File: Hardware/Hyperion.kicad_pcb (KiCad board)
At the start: 2 copper layers, 90.2 x 95.9 mm, 41 parts, among them J1 USB, J2 CONN-DC, Q1 MOSFET-P, Q2 FDC6561, U1 FT2232H, U2 93LC46/OT, U3 LTC4361-T, X1 12MHz

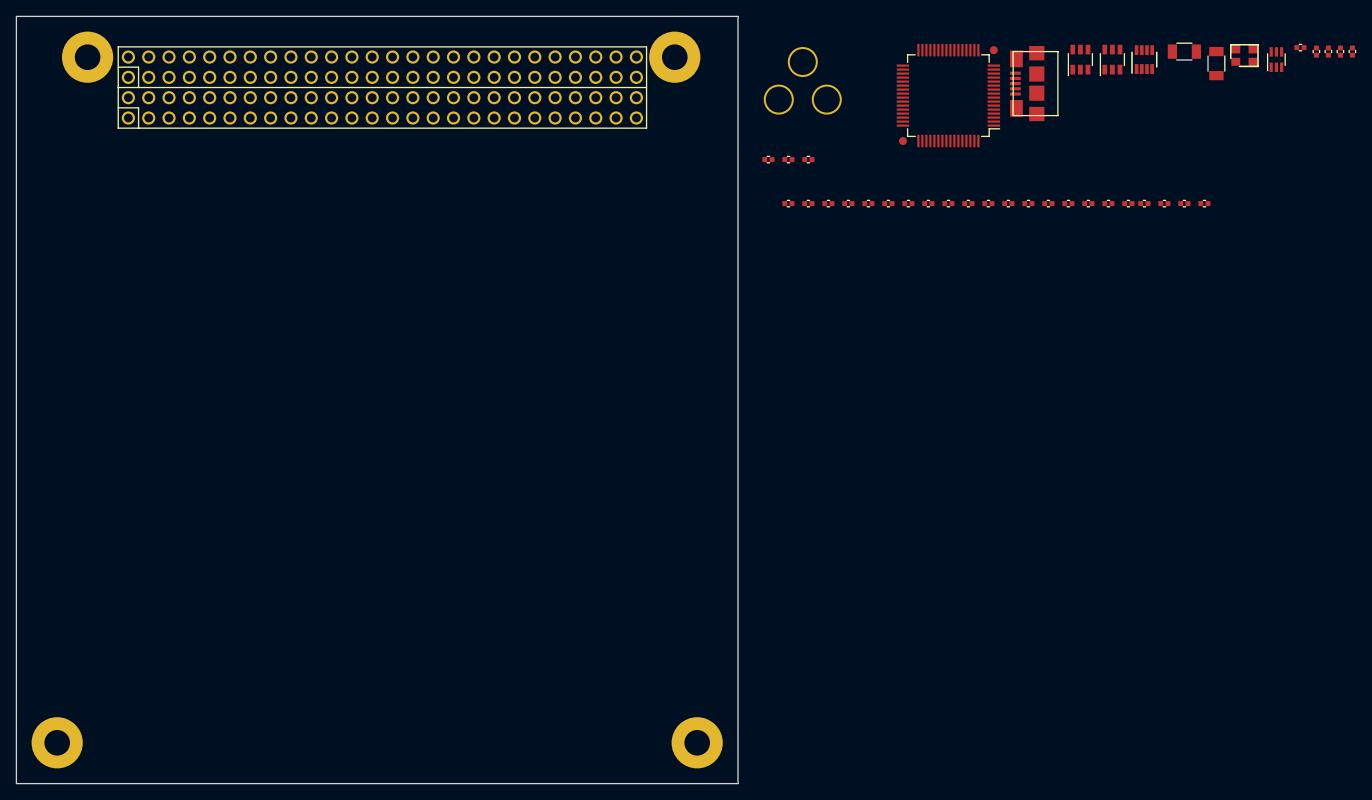
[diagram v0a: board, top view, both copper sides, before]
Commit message: Core support circuitry
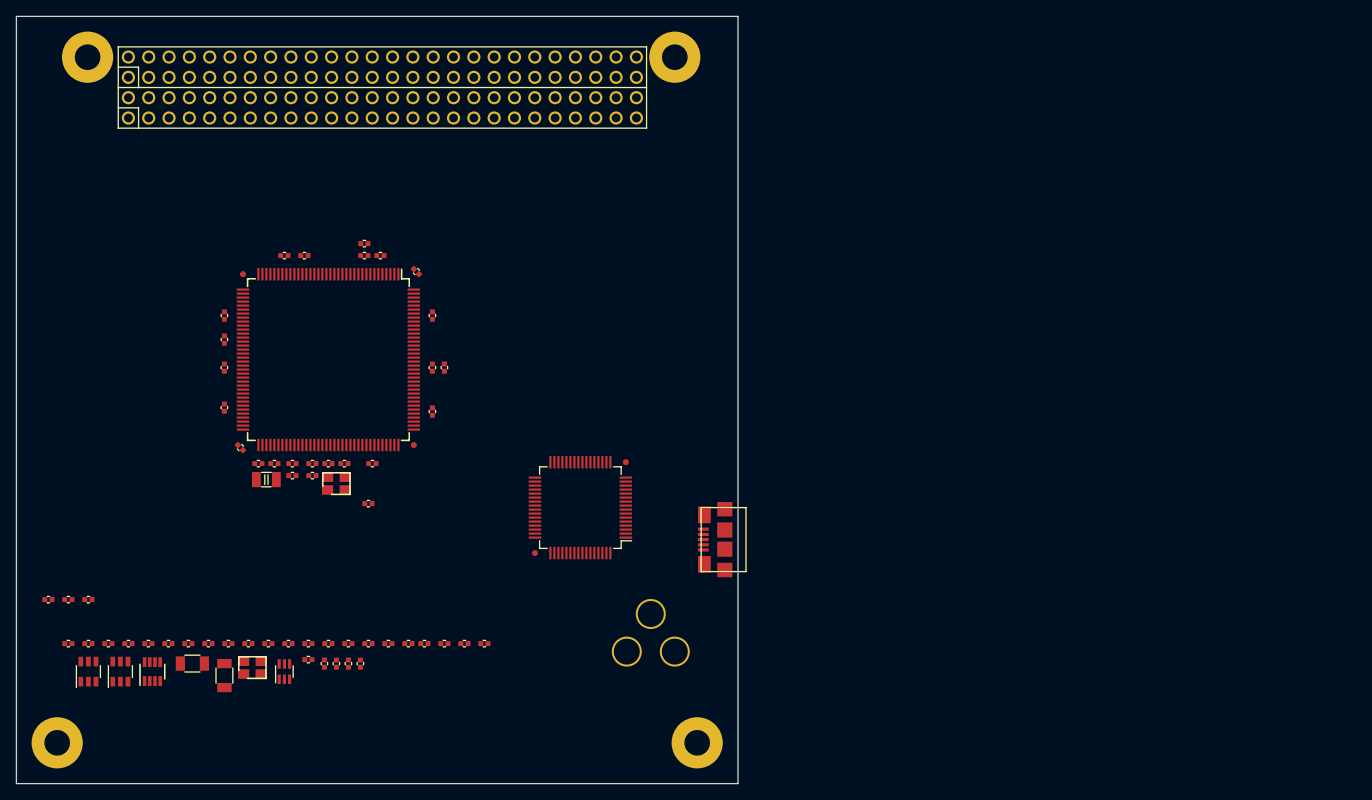
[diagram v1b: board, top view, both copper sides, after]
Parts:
- added C17: 0.1uF, CAPC1005-N, F.Cu at (145.5, 79.0)
- added C18: 0.1uF, CAPC1005-N, F.Cu at (136.0, 79.0)
- added C19: 0.1uF, CAPC1005-N, F.Cu at (133.5, 79.0)
- added C20: 0.1uF, CAPC1005-N, F.Cu at (126.0, 86.5)
- added C21: 0.1uF, CAPC1005-N, F.Cu at (126.0, 93.0)
- added C22: 0.1uF, CAPC1005-N, F.Cu at (126.0, 98.0)
- added C23: 0.1uF, CAPC1005-N, F.Cu at (134.5, 106.5)
- added C24: 0.1uF, CAPC1005-N, F.Cu at (144.0, 110.0)
- added C25: 0.1uF, CAPC1005-N, F.Cu at (144.5, 105.0)
- added C26: 0.1uF, CAPC1005-N, F.Cu at (152.0, 98.5)
- added C27: 0.1uF, CAPC1005-N, F.Cu at (152.0, 93.0)
- added C28: 0.1uF, CAPC1005-N, F.Cu at (152.0, 86.5)
- added C29: 3.3uF, CAPC1005-N, F.Cu at (150.0, 81.0)
- added C30: 3.3uF, CAPC1005-N, F.Cu at (128.0, 103.0)
- added C31: 0.1uF, CAPC1005-N, F.Cu at (126.0, 89.5)
- added C32: 3.3uF, CAPC1005-N, F.Cu at (153.5, 93.0)
- added C33: 10pF, CAPC1005-N, F.Cu at (139.0, 105.0)
- added C34: 10pF, CAPC1005-N, F.Cu at (130.2, 105.0)
- added C35: 10pF, CAPC1005-N, F.Cu at (141.0, 105.0)
- added C36: 10pF, CAPC1005-N, F.Cu at (132.2, 105.0)
- added C37: 0.1uF, CAPC1005-N, F.Cu at (143.5, 79.0)
- added C38: 0.1uF, CAPC1005-N, F.Cu at (134.5, 105.0)
- added C39: 0.1uF, CAPC1005-N, F.Cu at (137.0, 105.0)
- added FB3: FERRITE, INDC1005-N, F.Cu at (143.5, 77.5)
- added R12: 1k, RESC1005-N, F.Cu at (137.0, 106.5)
- added U4: TM4C123GH6PGE, QFP50P2200X2200-144N, F.Cu at (139.0, 92.0)
- added X2: 12MHz, XTAL-4SMD-32X25, F.Cu at (140.0, 107.5)
- added X3: 32.768kHz, XTAL-2SMD-32x15, F.Cu at (131.2, 107.0)
- C11, C14: value 27pF -> 10pF
- moved C16 145.7 mm to (136.5, 129.5)
- moved D1 145.7 mm to (141.5, 130.0)
- moved D2 145.7 mm to (143.0, 130.0)
- moved Q1 145.7 mm to (133.5, 131.0)
- moved Q2 145.7 mm to (109.0, 131.0)
- moved R1 145.7 mm to (138.5, 130.0)
- moved R11 145.7 mm to (122.0, 130.0)
- moved R2 145.7 mm to (140.0, 130.0)
- moved TH1 145.7 mm to (126.0, 131.5)
- moved U2 145.7 mm to (113.0, 131.0)
- moved U3 145.7 mm to (117.0, 131.0)
- moved X1 145.7 mm to (129.5, 130.5)
- moved C1 105.5 mm to (139.0, 127.5)
- moved C10 105.5 mm to (109.0, 127.5)
- moved C11 105.5 mm to (144.0, 127.5)
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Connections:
- H1 pad 1.42: (no net) -> VMEM
- U1 pad 16: (no net) -> /Core/TCK
- U1 pad 17: (no net) -> /Core/TDI
- U1 pad 18: (no net) -> /Core/TDO
- U1 pad 19: (no net) -> /Core/TMS
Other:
- copper layers 2 -> 4
- net class Default: clearance 0.2032 -> 0.1524; trace_width 0.2032 -> 0.1524; via_dia 0.889 -> 0.4572; via_drill 0.635 -> 0.254
- rule trace_clearance: 0.2032 -> 0.1524
- rule trace_min: 0.1524 -> 0.127
- rule via_min_drill: 0.508 -> 0.254
- rule via_min_size: 0.889 -> 0.4572

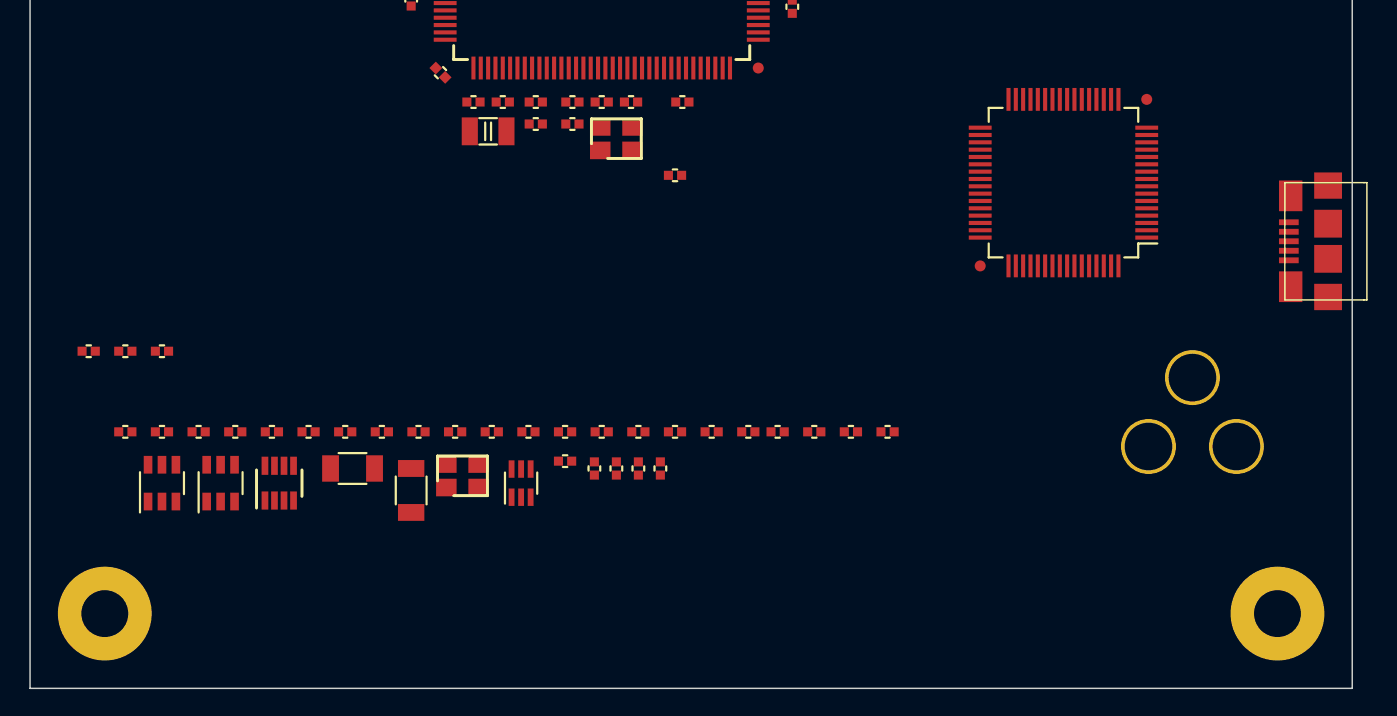
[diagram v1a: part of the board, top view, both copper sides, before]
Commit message: Rough layout
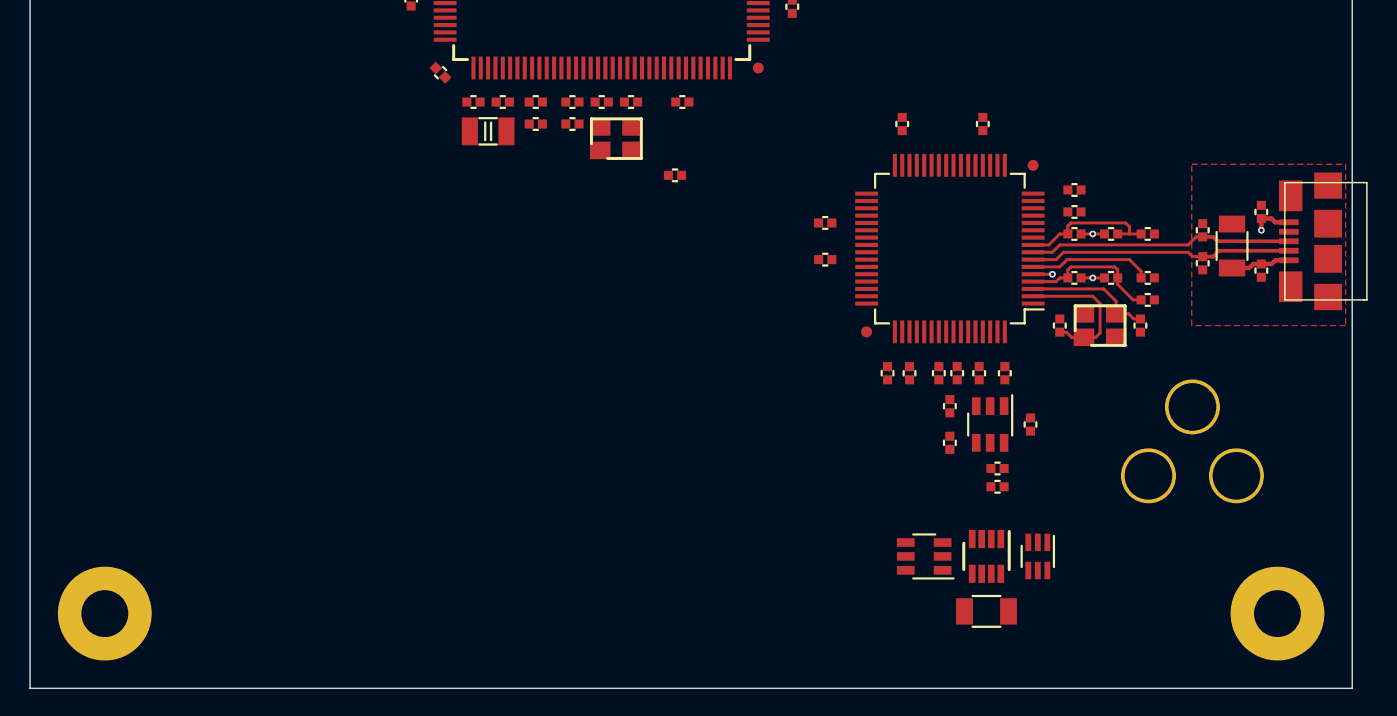
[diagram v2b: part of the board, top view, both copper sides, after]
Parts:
- moved R3 70.5 mm to (176.2, 117.0), turned to 180 degrees
- moved R5 60.8 mm to (164.8, 123.5), turned to 270 degrees
- moved TH1 58.4 mm to (182.0, 114.8), turned to 270 degrees
- moved R7 56.4 mm to (162.8, 125.8), turned to 270 degrees
- moved R10 54.1 mm to (162.8, 128.2), turned to 270 degrees
- moved C10 53.2 mm to (162.0, 123.5), turned to 270 degrees
- moved C7 52.9 mm to (165.0, 106.5), turned to 90 degrees
- moved U2 52.7 mm to (165.5, 127.0), turned to 180 degrees
- moved Q2 52.2 mm to (161.0, 136.0), turned to 90 degrees
- moved C4 50.8 mm to (171.2, 117.0)
- moved C8 50.1 mm to (159.5, 106.5), turned to 90 degrees
- moved C2 49.1 mm to (171.2, 114.0)
- moved U3 48.5 mm to (165.2, 136.0), turned to 180 degrees
- moved R1 47.5 mm to (184.0, 116.5)
- moved R2 47.4 mm to (184.0, 112.5)
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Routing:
- net /Interface Port/D+: track 0.00 -> 18.0 mm
- net /Interface Port/D-: track 0.00 -> 17.9 mm
- net /Interface Port/OSCI: track 0.00 -> 9.80 mm
- net N-00000109: track 0.00 -> 9.72 mm
- net N-00000108: track 0.00 -> 9.62 mm
- net /Interface Port/OSCO: track 0.00 -> 8.67 mm
- net N-00000101: track 0.00 -> 8.36 mm
- net GND: track 0.00 -> 7.30 mm, vias 0 -> 4
- net N-00000105: track 0.00 -> 4.09 mm
- added copper zone on F.Cu, net /Interface Port/Shield
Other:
- net class USB added: clearance 0.2032, trace_width 0.254, via_dia 0.4572, via_drill 0.254
